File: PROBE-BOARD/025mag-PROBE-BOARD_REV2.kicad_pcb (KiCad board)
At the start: 2 copper layers, 15 x 26.7 mm, 12 parts, among them M31 MountingHole_3.2mm_M3, SW1 SW_Push_Open

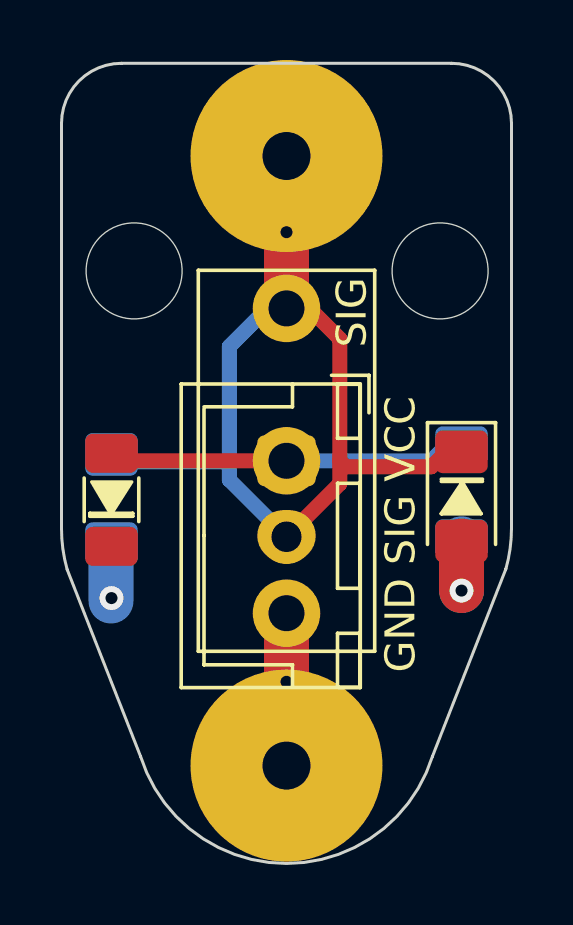
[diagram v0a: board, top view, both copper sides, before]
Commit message: ADDED VIAS
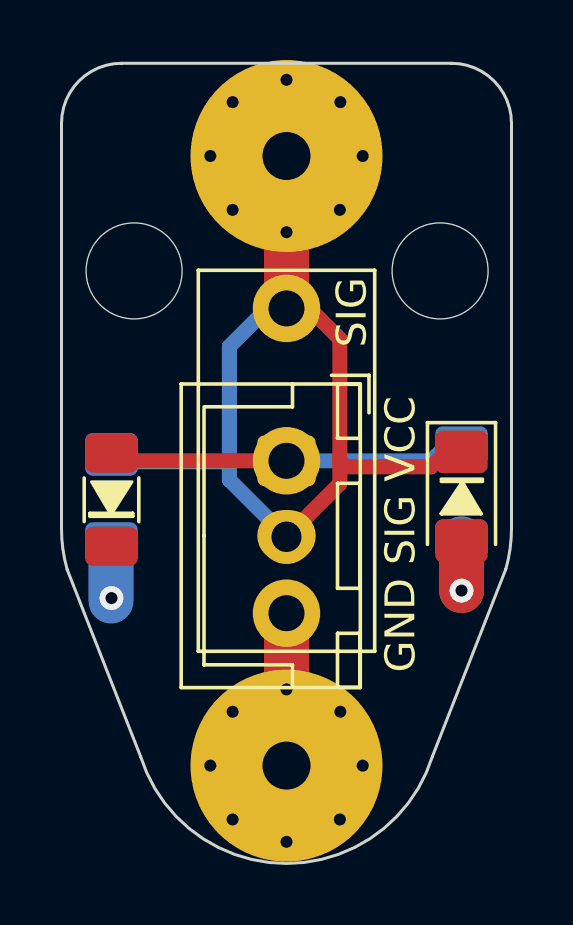
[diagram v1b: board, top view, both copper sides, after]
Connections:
- REF** pad 2: (no net) -> SIGNAL
- REF** pad 3: (no net) -> GND
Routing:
- net SIGNAL: vias 1 -> 8
- net GND: vias 1 -> 8
